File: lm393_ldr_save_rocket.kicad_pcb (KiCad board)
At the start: 2 copper layers, 50 x 50 mm, 18 parts, among them J1 BAT 9V, J2 IGNITER, J3 JUMP, M3 M3, Q2 TIP120, U1 LM7805, U2 LM393

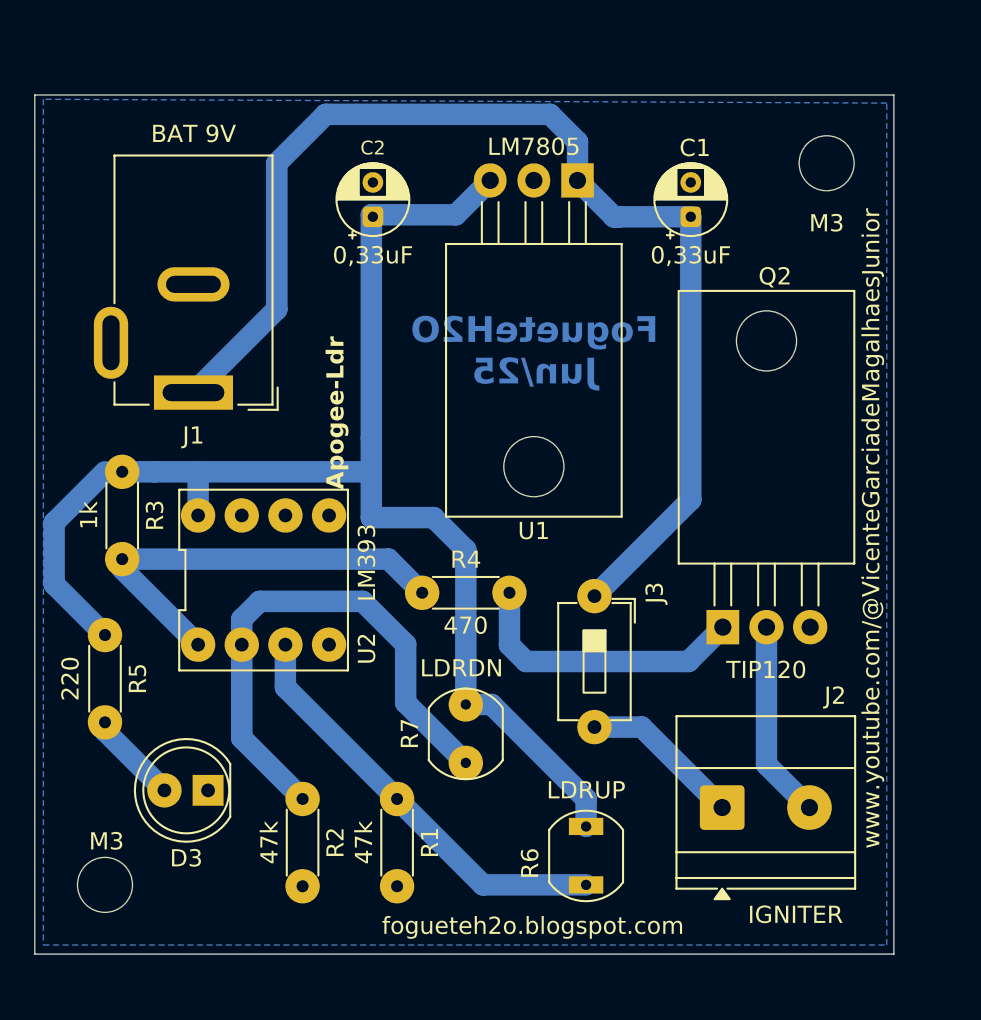
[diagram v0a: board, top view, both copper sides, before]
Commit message: finalizada com order para JCLPCB
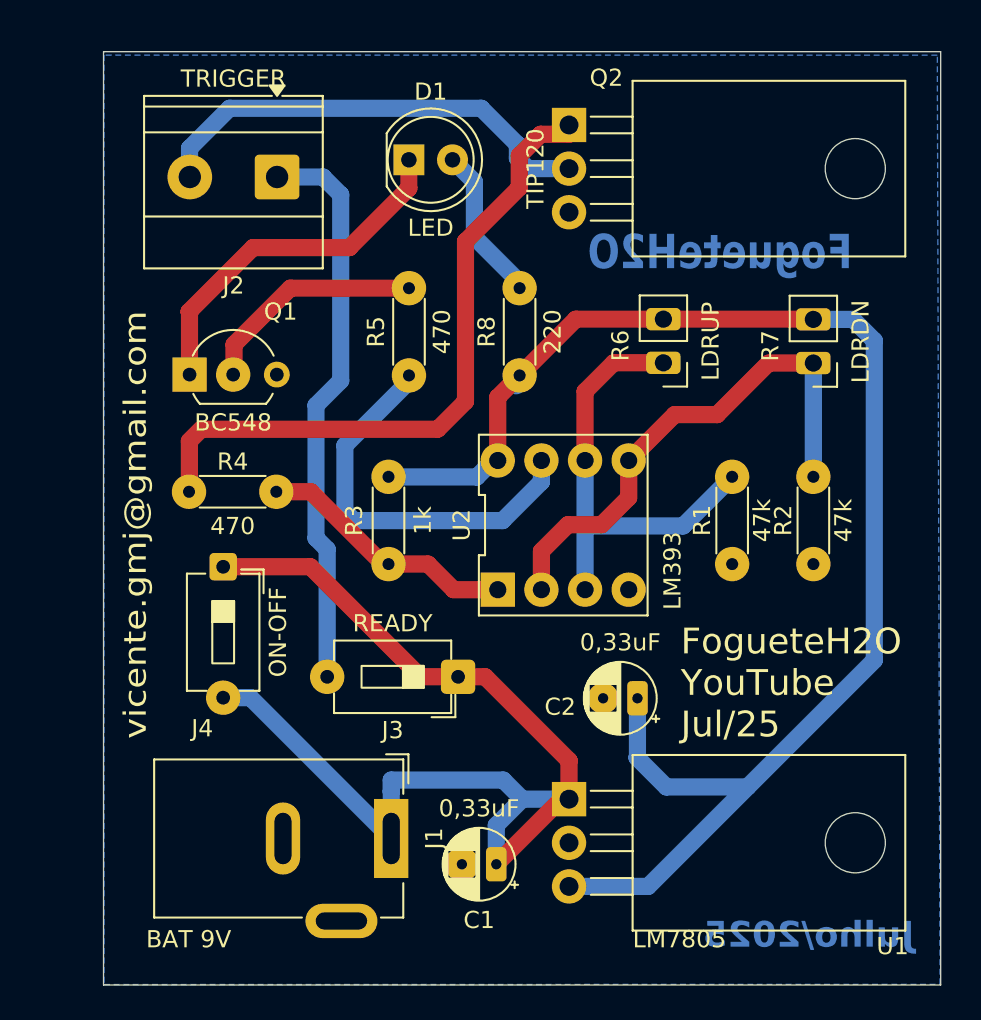
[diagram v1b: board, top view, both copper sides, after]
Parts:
- removed D3: LED, LED_THT:LED_D5.0mm
- removed M3 (x2): M3, MountingHole:MountingHole_3.2mm_M3
- added D1: LED, LED_THT:LED_D5.0mm, F.Cu at (106.7, 67.3)
- added J4: ON-OFF, Button_Switch_THT:SW_DIP_SPSTx01_Slide_6.7x4.1mm_W7.62mm_P2.54mm_LowProfile, F.Cu at (95.9, 91.0)
- added Q1: BC548, Package_TO_SOT_THT:TO-92L_Inline_Wide, F.Cu at (93.9, 79.8)
- added R8: 220, Resistor_THT:R_Axial_DIN0204_L3.6mm_D1.6mm_P5.08mm_Horizontal, F.Cu at (113.1, 79.8)
- J2: value IGNITER -> TRIGGER
- J3: value JUMP -> READY
- R5: value 220 -> 470
- R6, R7: footprint OptoDevice:R_LDR_5.1x4.3mm_P3.4mm_Vertical -> Connector_PinHeader_2.54mm:PinHeader_1x02_P2.54mm_Vertical
- moved J2 44.9 mm to (99.0, 68.3), turned to 180 degrees
- moved C1 39.3 mm to (111.8, 108.3), turned to 180 degrees
- moved U1 36.0 mm to (116.0, 104.5), turned to -90 degrees
- moved R2 35.1 mm to (130.2, 85.8)
- moved C2 32.0 mm to (120.0, 98.6), turned to 180 degrees
- moved R7 30.8 mm to (130.2, 79.1), turned to 180 degrees
- moved R6 30.7 mm to (121.5, 79.1), turned to 180 degrees
- moved Q2 30.6 mm to (116.0, 65.3), turned to -90 degrees
- moved J1 28.4 mm to (105.7, 106.8), turned to -90 degrees
- moved R1 27.1 mm to (125.5, 85.8)
- moved R5 23.3 mm to (106.7, 79.8), turned to 90 degrees
- moved U2 17.7 mm to (115.7, 88.6)
- moved R3 15.5 mm to (105.5, 85.8)
- moved R4 10.3 mm to (99.0, 86.6), turned to 180 degrees
- moved J3 9.22 mm to (109.5, 97.4), turned to 180 degrees
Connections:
- C1 pad 1: Net-(J1-Pin_1) -> Net-(J3-Pin_1)
- J3 pad 1: Net-(J1-Pin_1) -> Net-(J3-Pin_1)
- R5 pad 1: /VCC -> Net-(R5-Pad1)
- U1 pad 1: Net-(J1-Pin_1) -> Net-(J3-Pin_1)
- U2 pad 5: (no net) -> Net-(U2A--)
- U2 pad 6: (no net) -> Net-(U2A-+)
- U2 pad 7: (no net) -> Net-(R5-Pad1)
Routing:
- net Net-(J1-Pin_1): track 68.8 -> 32.8 mm
- net Net-(J3-Pin_1): track 0.00 -> 32.9 mm
- net Net-(J2-Pin_1): track 9.37 -> 33.6 mm
- net Net-(R5-Pad1): track 0.00 -> 22.7 mm
- net Net-(Q2-B): track 16.7 -> 38.7 mm
- net Net-(D1-K): track 0.00 -> 21.1 mm
- net Net-(J2-Pin_2): track 11.5 -> 26.6 mm
- net Net-(R3-Pad2): track 25.6 -> 15.3 mm
- net Net-(D1-A): track 0.00 -> 9.47 mm
- net Net-(Q1-B): track 5.39 -> 13.3 mm
- net /VCC: track 80.6 -> 86.7 mm
- net Net-(U2A-+): track 24.7 -> 26.5 mm
- net Net-(U2A--): track 31.3 -> 30.6 mm
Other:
- board size 50 x 50 mm -> 48.7 x 54.3 mm
- board text added: "FogueteH2O"
- board text added: "FogueteH2O YouTube Jul/25"
- board text added: "Julho/2025"
- board text added: "vicente.gmj@gmail.com"
- board text removed: "Apogee-Ldr"
- board text removed: "FogueteH2O Jun/25"
- board text removed: "fogueteh2o.blogspot.com"
- board text removed: "www.youtube.com/@VicenteGarciadeMagalhaesJunior"
